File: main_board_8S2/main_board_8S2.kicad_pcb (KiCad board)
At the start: 2 copper layers, 114.3 x 86.4 mm, 47 parts

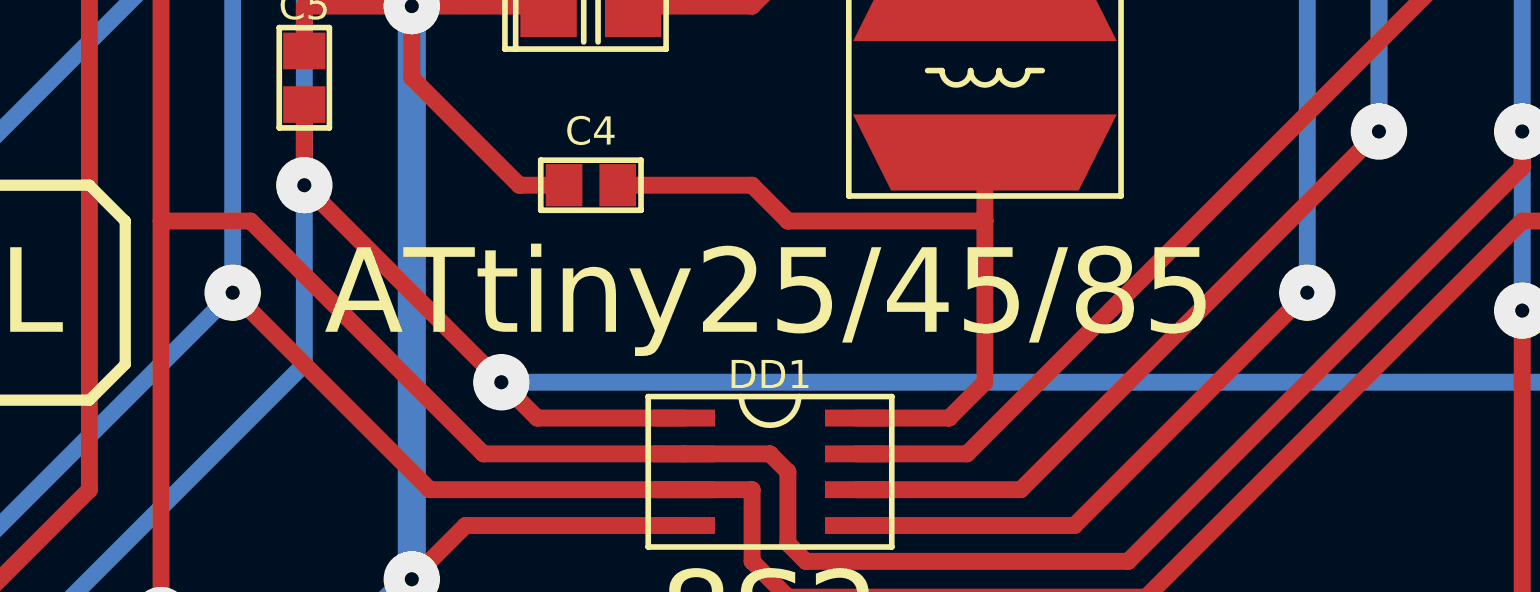
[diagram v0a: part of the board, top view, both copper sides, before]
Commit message: Обновлены УГО ИМС
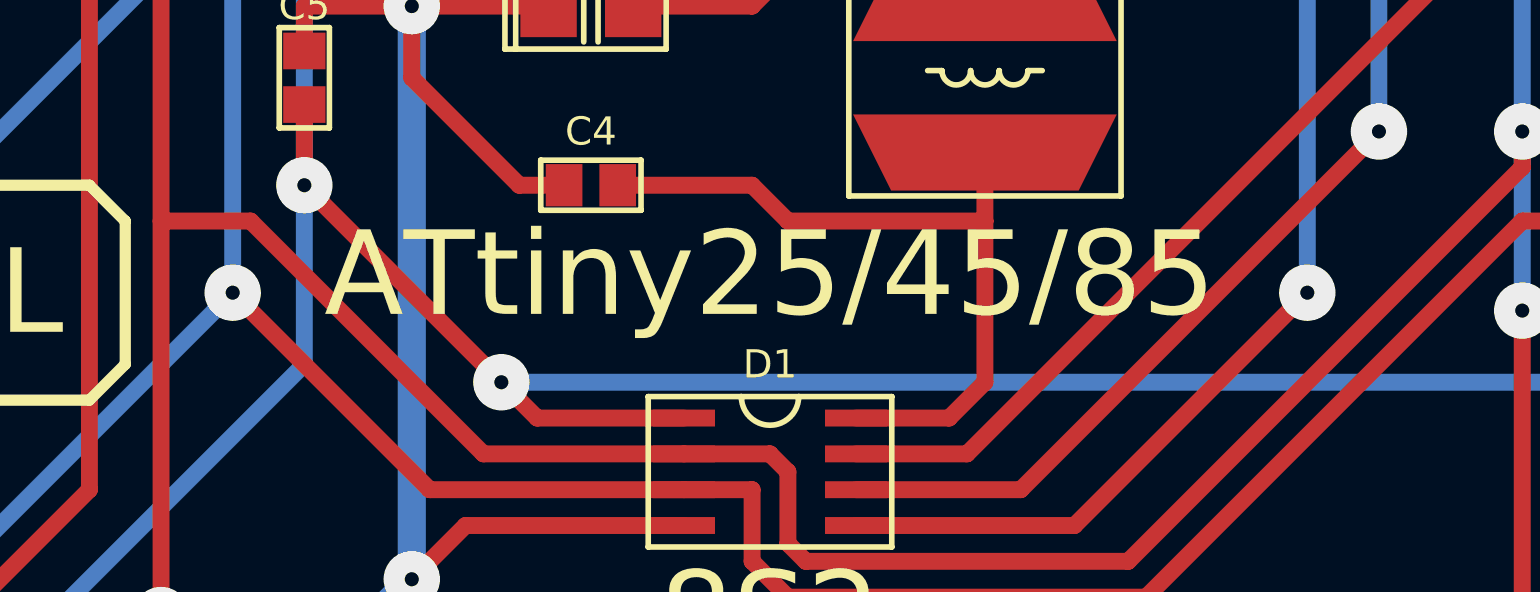
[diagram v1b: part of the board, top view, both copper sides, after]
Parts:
- removed DD1: IC_MCU_AVR_TINY_25-45-85_8S2, KCL:P-SO-08A
- added D1: ATtiny25-20SU, KCL:P-SO-08A, F.Cu at (148.6, 104.1)
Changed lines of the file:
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@@
-(kicad_pcb (version 20171130) (host pcbnew 5.0.0-fee4fd1~66~ubuntu18.04.1)
+(kicad_pcb (version 20171130) (host pcbnew 5.0.2-bee76a0~70~ubuntu18.04.1)
   (general
     (thickness 1.5)
@@
   (title_block
     (title main_board_8S2)
-    (date 2019-02-18)
+    (date 2019-05-15)
     (rev 1)
     (company "Igor Vladimirovich Ivanov")
@@
     (pad_drill 0.762)
     (pad_to_mask_clearance 0.2)
+    (solder_mask_min_width 0.25)
     (aux_axis_origin 0 0)
     (visible_elements 7FFFFFFF)
@@
     (at 148.59 104.14)
     (attr smd)
-    (fp_text reference DD1 (at 0 -3.429) (layer F.SilkS)
-      (effects (font (size 1 1) (thickness 0.2)))
-    )
-    (fp_text value IC_MCU_AVR_TINY_25-45-85_8S2 (at 0 -4.699) (layer F.Fab) hide
+    (fp_text reference D1 (at 0 -3.81) (layer F.SilkS)
+      (effects (font (size 1 1) (thickness 0.2)))
+    )
+    (fp_text value ATtiny25-20SU (at 10.16 0) (layer F.Fab) hide
       (effects (font (size 1 1) (thickness 0.2)))
     )
@@
   (gr_line (start 205.74 60.96) (end 205.74 147.32) (angle 90) (layer Edge.Cuts) (width 0.4))
   (gr_line (start 91.44 60.96) (end 205.74 60.96) (angle 90) (layer Edge.Cuts) (width 0.4))
-  (gr_text ATtiny25/45/85 (at 148.59 97.79) (layer F.SilkS)
+  (gr_text ATtiny25/45/85 (at 148.59 97.155) (layer F.SilkS)
     (effects (font (size 3 3) (thickness 0.6)))
   )
